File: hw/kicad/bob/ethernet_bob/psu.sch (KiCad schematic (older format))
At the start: 12 parts, among them U3 LM3578

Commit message: Yes yes git and the like.
Fix crystal symbol
Add flash
Add Vreg
Add USB-A

Still WIP...
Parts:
- removed C17, C18: 18pF, Capacitors_SMD:C_0603, symbol C
- removed C19: 1nF, Capacitors_SMD:C_0603, symbol C
- removed D1: D_Schottky, Diodes_SMD:SOD-123, symbol D_Schottky
- removed D2: LED, LEDs:LED_0603, symbol LED
- removed L1: INDUCTOR_SMALL, Inductors_NEOSID:Neosid_Inductor_Ms85, symbol INDUCTOR_SMALL
- removed R11, R7, R8: R, Resistors_SMD:R_0603, symbol R
- removed R9: 1, Resistors_SMD:R_0805, symbol R
- removed U3: LM3578, Housings_SOIC:SOIC-8_3.9x4.9mm_Pitch1.27mm, symbol LM3578
- added C21: C, Capacitors_SMD:C_0603, symbol C
- added U3: NCP1117ST33T3G, TO_SOT_Packages_SMD:SOT-223, symbol NCP1117ST33T3G
- C20: value 220µF -> C; footprint Capacitors_SMD:C_1206 -> Capacitors_SMD:C_0603
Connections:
- net labels added: +3.3V, +5VP
- net labels removed: +24V, +3V3
- wire segments 16 -> 4

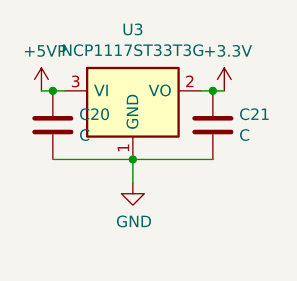
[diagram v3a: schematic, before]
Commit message: More stuff
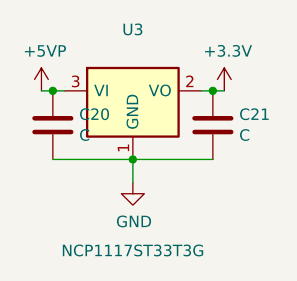
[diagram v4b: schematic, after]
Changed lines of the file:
@@
 $Descr A4 11693 8268
 encoding utf-8
-Sheet 4 6
+Sheet 3 6
 Title ""
 Date ""
@@
 $EndDescr
 $Comp
-L GND #PWR15
+L GND #PWR018
 U 1 1 57FEA6D9
 P 6300 3500
-F 0 "#PWR15" H 6300 3250 50  0001 C CNN
+F 0 "#PWR018" H 6300 3250 50  0001 C CNN
 F 1 "GND" H 6305 3327 50  0000 C CNN
 F 2 "" H 6300 3500 50  0000 C CNN
@@
 $EndComp
 $Comp
-L +3.3V #PWR16
+L +3.3V #PWR019
 U 1 1 57FEA6EF
 P 6700 3100
-F 0 "#PWR16" H 6700 2950 50  0001 C CNN
+F 0 "#PWR019" H 6700 2950 50  0001 C CNN
 F 1 "+3.3V" H 6715 3273 50  0000 C CNN
 F 2 "" H 6700 3100 50  0000 C CNN
@@
 $EndComp
 $Comp
-L +5VP #PWR14
+L +5VP #PWR020
 U 1 1 57FEA707
 P 5900 3100
-F 0 "#PWR14" H 5900 2950 50  0001 C CNN
+F 0 "#PWR020" H 5900 2950 50  0001 C CNN
 F 1 "+5VP" H 5915 3273 50  0000 C CNN
 F 2 "" H 5900 3100 50  0000 C CNN
@@
 P 6300 3100
 F 0 "U3" H 6300 3367 50  0000 C CNN
-F 1 "NCP1117ST33T3G" H 6300 3276 50  0000 C CNN
+F 1 "NCP1117ST33T3G" H 6300 2400 50  0000 C CNN
 F 2 "TO_SOT_Packages_SMD:SOT-223" H 6350 2850 50  0001 L CNN
 F 3 "" H 6300 3100 50  0000 C CNN

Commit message: netbob lables
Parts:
- C20, C21: footprint Capacitors_SMD:C_0603 -> stmbl:C_0603
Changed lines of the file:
@@
 EESchema Schematic File Version 2
-LIBS:ethernet_bob-rescue
 LIBS:power
 LIBS:device
@@
 LIBS:usblc
 LIBS:ethernet_bob-cache
-EELAYER 25 0
+EELAYER 26 0
 EELAYER END
 $Descr A4 11693 8268
@@
 $EndDescr
 $Comp
-L GND #PWR20
+L GND #PWR019
 U 1 1 57FEA6D9
 P 6300 3500
-F 0 "#PWR20" H 6300 3250 50  0001 C CNN
+F 0 "#PWR019" H 6300 3250 50  0001 C CNN
 F 1 "GND" H 6305 3327 50  0000 C CNN
 F 2 "" H 6300 3500 50  0000 C CNN
@@
 $EndComp
 $Comp
-L +3.3V #PWR21
+L +3.3V #PWR020
 U 1 1 57FEA6EF
 P 6700 3100
-F 0 "#PWR21" H 6700 2950 50  0001 C CNN
+F 0 "#PWR020" H 6700 2950 50  0001 C CNN
 F 1 "+3.3V" H 6715 3273 50  0000 C CNN
 F 2 "" H 6700 3100 50  0000 C CNN
@@
 $EndComp
 $Comp
-L +5VP #PWR19
+L +5VP #PWR021
 U 1 1 57FEA707
 P 5900 3100
-F 0 "#PWR19" H 5900 2950 50  0001 C CNN
+F 0 "#PWR021" H 5900 2950 50  0001 C CNN
 F 1 "+5VP" H 5915 3273 50  0000 C CNN
 F 2 "" H 5900 3100 50  0000 C CNN
@@
 F 0 "C20" H 6065 3296 50  0000 L CNN
 F 1 "C" H 6065 3205 50  0000 L CNN
-F 2 "Capacitors_SMD:C_0603" H 5988 3100 50  0001 C CNN
+F 2 "stmbl:C_0603" H 5988 3100 50  0001 C CNN
 F 3 "" H 5950 3250 50  0000 C CNN
 	1    5950 3250
@@
 F 0 "C21" H 6765 3296 50  0000 L CNN
 F 1 "C" H 6765 3205 50  0000 L CNN
-F 2 "Capacitors_SMD:C_0603" H 6688 3100 50  0001 C CNN
+F 2 "stmbl:C_0603" H 6688 3100 50  0001 C CNN
 F 3 "" H 6650 3250 50  0000 C CNN
 	1    6650 3250
